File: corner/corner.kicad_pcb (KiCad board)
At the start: 2 copper layers, 50 x 50 mm, 7 parts, among them J1 Conn_01x02, J2 Conn_01x02, J3 Conn_01x02, J4 Conn_01x02

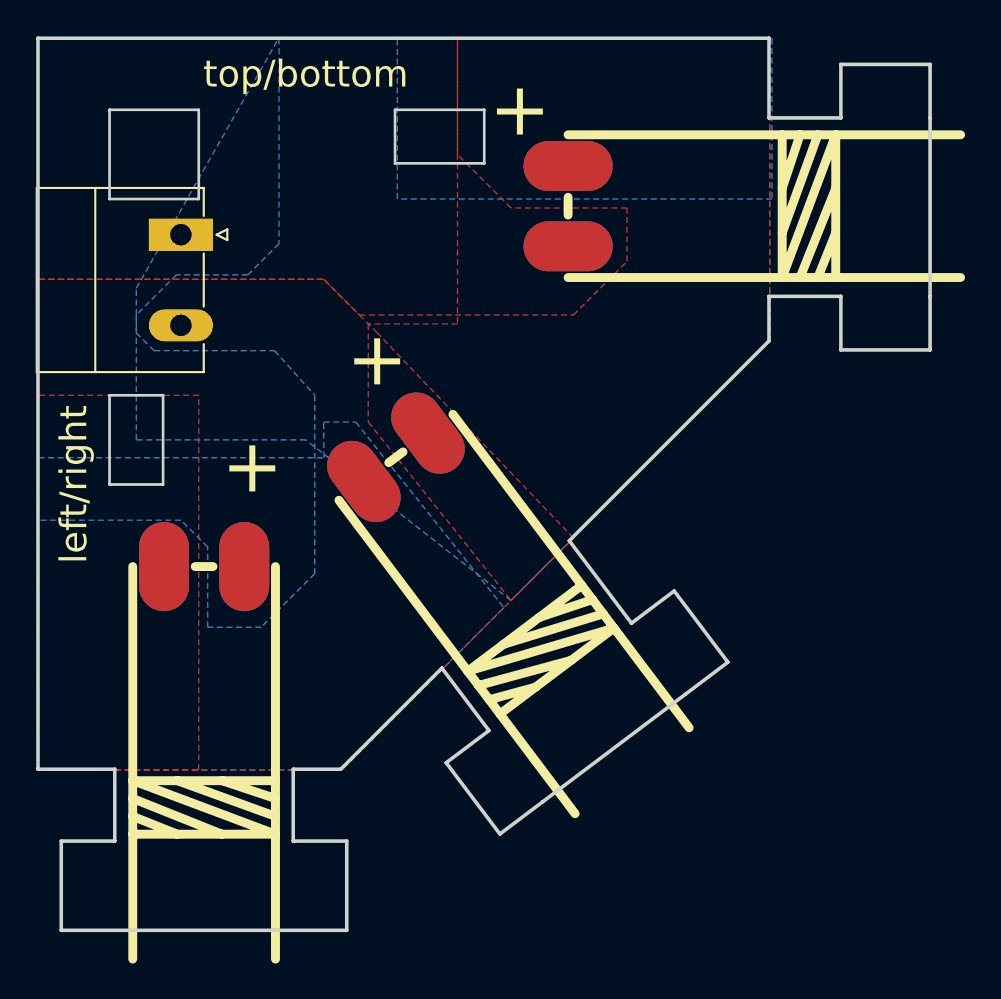
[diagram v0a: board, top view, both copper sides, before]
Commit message: PCB designs R01 finished (not reviewed yet)
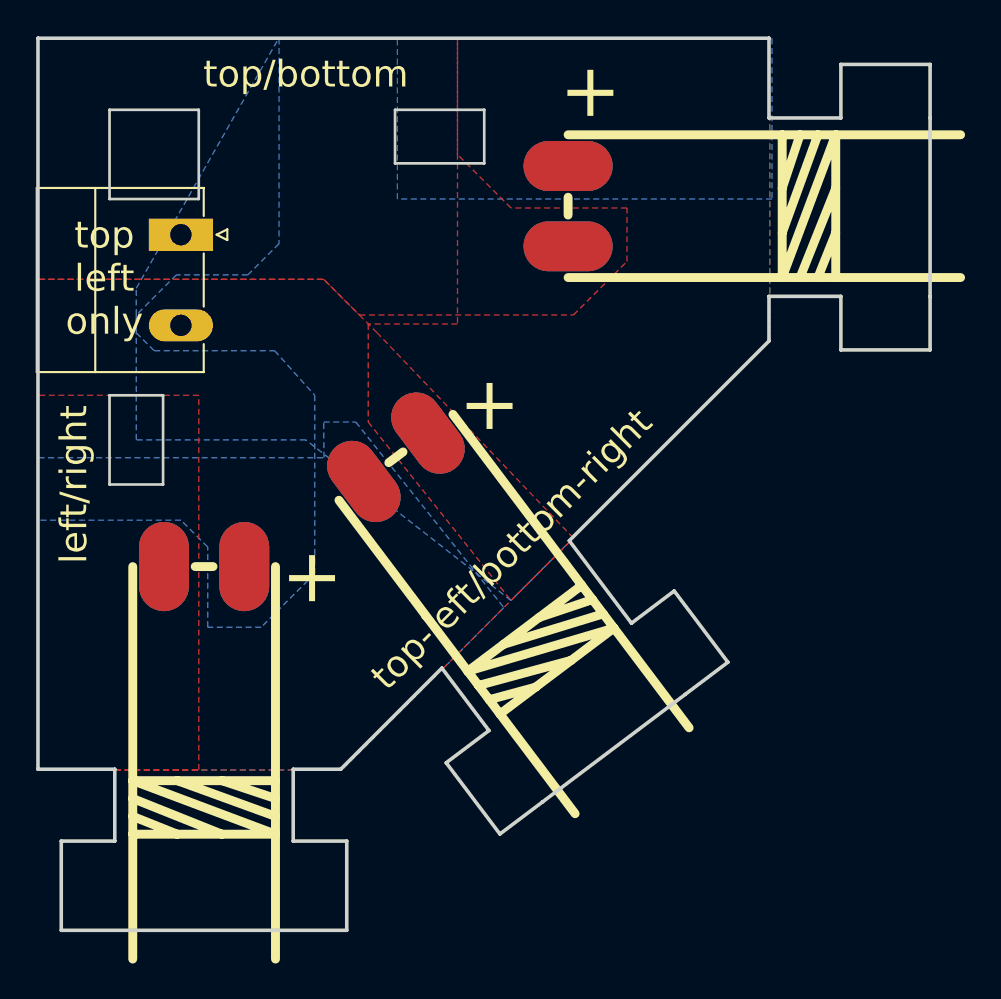
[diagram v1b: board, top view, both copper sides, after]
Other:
- board text added: "(c)2018 jaseg"
- board text added: "8seg R01"
- board text added: "bottom-left/top-right"
- board text added: "cc-by-sa"
- board text added: "github.com/jaseg/8seg"
- board text added: "top left only"
- board text added: "top-left/bottom-right"
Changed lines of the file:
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@@
   (general
     (thickness 1.6)
-    (drawings 55)
+    (drawings 62)
     (tracks 0)
     (zones 0)
@@
       (net 4 /D))
   )
-  (gr_text left/right (at 147 49 90) (layer B.SilkS)
+  (gr_text github.com/jaseg/8seg (at 146.8 61.72 90) (layer B.SilkS)
+    (effects (font (size 1.5 1.5) (thickness 0.3)) (justify mirror))
+  )
+  (gr_text cc-by-sa (at 163.5 44.7 90) (layer B.SilkS)
+    (effects (font (size 1.5 1.5) (thickness 0.3)) (justify mirror))
+  )
+  (gr_text "(c)2018 jaseg" (at 161.01 46.74 90) (layer B.SilkS)
+    (effects (font (size 1.5 1.5) (thickness 0.3)) (justify mirror))
+  )
+  (gr_text "8seg R01" (at 157.22 49.73 90) (layer B.SilkS)
+    (effects (font (size 3 3) (thickness 0.6)) (justify mirror))
+  )
+  (gr_text "top\nleft\nonly" (at 148.71 48.44) (layer F.SilkS)
+    (effects (font (size 1.5 1.5) (thickness 0.3)))
+  )
+  (gr_text bottom-left/top-right (at 171.6 63.49 45) (layer B.SilkS)
+    (effects (font (size 1.5 1.5) (thickness 0.3)) (justify mirror))
+  )
+  (gr_text top-left/bottom-right (at 171.53 63.63 45) (layer F.SilkS)
+    (effects (font (size 1.5 1.5) (thickness 0.3)))
+  )
+  (gr_text left/right (at 146.8 41.69 90) (layer B.SilkS)
     (effects (font (size 1.5 1.5) (thickness 0.3)) (justify mirror))
   )
@@
     (effects (font (size 3 3) (thickness 0.75)) (justify mirror))
   )
-  (gr_text + (at 160 56) (layer B.SilkS)
+  (gr_text + (at 161.04 64.38) (layer B.SilkS)
     (effects (font (size 3 3) (thickness 0.75)) (justify mirror))
   )
-  (gr_text + (at 169 47) (layer B.SilkS)
+  (gr_text + (at 176.57 50.14) (layer B.SilkS)
     (effects (font (size 3 3) (thickness 0.75)) (justify mirror))
   )
-  (gr_text + (at 164 53) (layer F.SilkS)
+  (gr_text + (at 170.3 55.5) (layer F.SilkS)
     (effects (font (size 3 3) (thickness 0.75)))
   )
-  (gr_text + (at 157 59) (layer F.SilkS)
+  (gr_text + (at 160.35 65.15) (layer F.SilkS)
     (effects (font (size 3 3) (thickness 0.75)))
   )
-  (gr_text + (at 172 39) (layer F.SilkS)
+  (gr_text + (at 175.95 37.95) (layer F.SilkS)
     (effects (font (size 3 3) (thickness 0.75)))
   )
